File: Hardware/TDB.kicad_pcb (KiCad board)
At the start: 2 copper layers, 47 parts, among them J1 RJ45_CANBUS, J10 Conn_01x02_Male, J11 Conn_01x02_Male, J12 Conn_01x02_Male, J18 Conn_01x01_Female, J2 Conn_01x03_Female_Potar, J21 Conn_01x01_Female, J22 Conn_01x01_Female, J3 Conn_01x03_Female_Servomotor, J4 Conn_01x02_Female, J5 Conn_01x02_Female, J6 Conn_01x02_Female, J7 Conn_01x02_Female, J8 Conn_01x03_Female, J9 Conn_01x02_Male, Q1 IRFZ44Z, Q2 IRFZ44Z, U1 MOLEX_SABRE_46007-1102, U2 L7805, U3 L7805, U4 L7812, U5 MCP2551-I-SN, U6 TC4424, U7 STM32H103-OlimexBoard

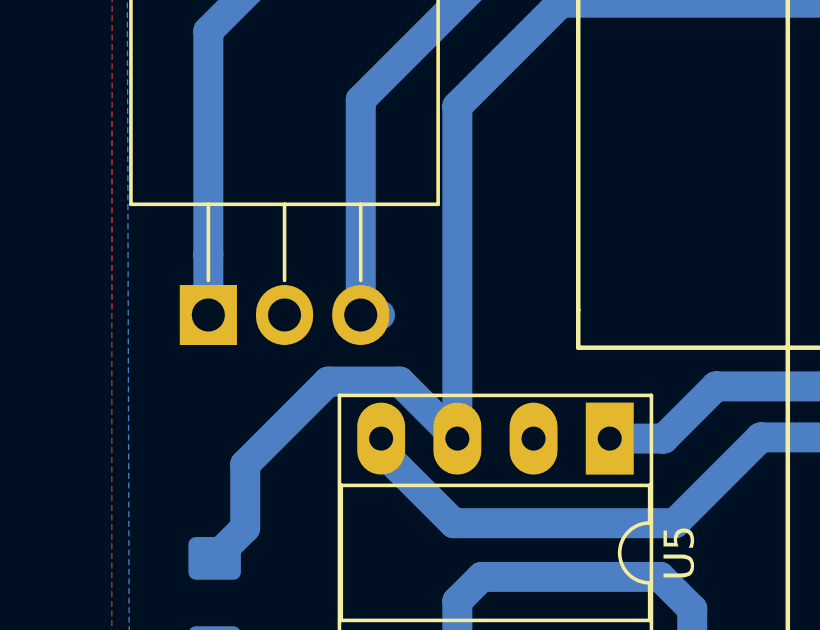
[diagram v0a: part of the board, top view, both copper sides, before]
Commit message: Re-master workstation : Put every relatade files together
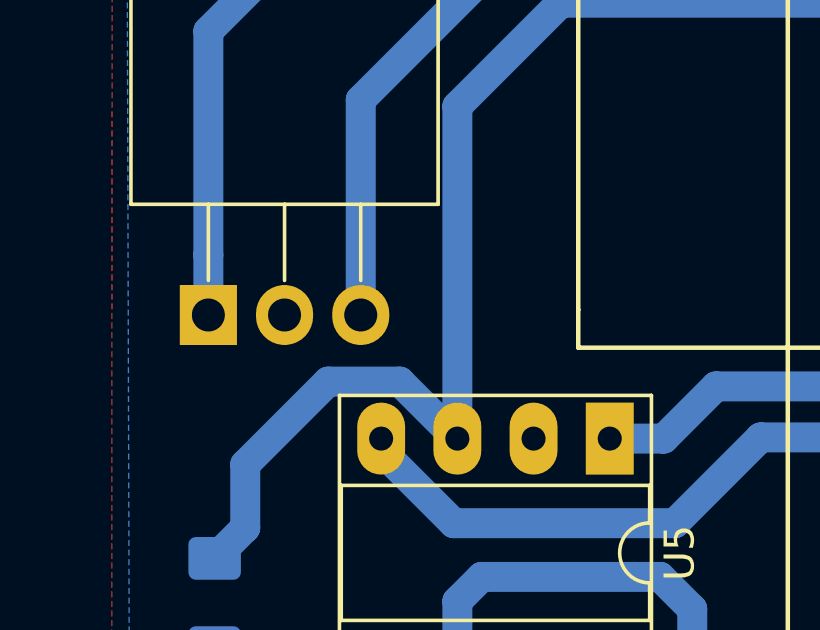
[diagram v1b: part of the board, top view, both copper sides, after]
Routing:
- net (no net): track 967.0 -> 966.3 mm
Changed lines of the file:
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@@
     (thickness 1.6)
     (drawings 9)
-    (tracks 232)
+    (tracks 231)
     (zones 0)
     (modules 47)
@@
     (solder_mask_min_width 0.25)
     (aux_axis_origin 0 0)
-    (visible_elements FFFFFF7F)
+    (visible_elements 7FFFFFFF)
     (pcbplotparams
       (layerselection 0x010fc_ffffffff)
@@
   (segment (start 135.789999 93.509999) (end 134.92 94.379998) (width 1) (layer B.Cu) (net 0))
   (segment (start 137.06 92.66) (end 136.210001 93.509999) (width 1) (layer B.Cu) (net 0))
-  (segment (start 119.01 110) (end 119.6525 110) (width 1) (layer B.Cu) (net 0))
   (segment (start 136.210001 93.509999) (end 135.789999 93.509999) (width 1) (layer B.Cu) (net 0))
   (segment (start 134.92 95.95102) (end 133.74102 97.13) (width 1) (layer B.Cu) (net 0))

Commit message: Beta version. all functions are working and are tested. - break (CAN msg on rise and fall) - wiper control - fan - Front light and back light the code still need to be organize and commented.
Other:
- board text added: "-26 to get the right pin number from H103 Doc"
- board text added: "BREAK_SW"
- board text added: "CLIM_SW"
- board text added: "FAN"
- board text added: "Front Back"
- board text added: "Head Light"
- board text added: "WIPER"
- board text added: "WIPER_SPEED"
